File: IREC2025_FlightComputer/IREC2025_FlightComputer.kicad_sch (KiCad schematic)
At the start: 36 parts, among them J1 Molex Microfit, U1 STM32U575VGTx, U2 TPS62153, U3 LP5912Q3.3DRVRQ1

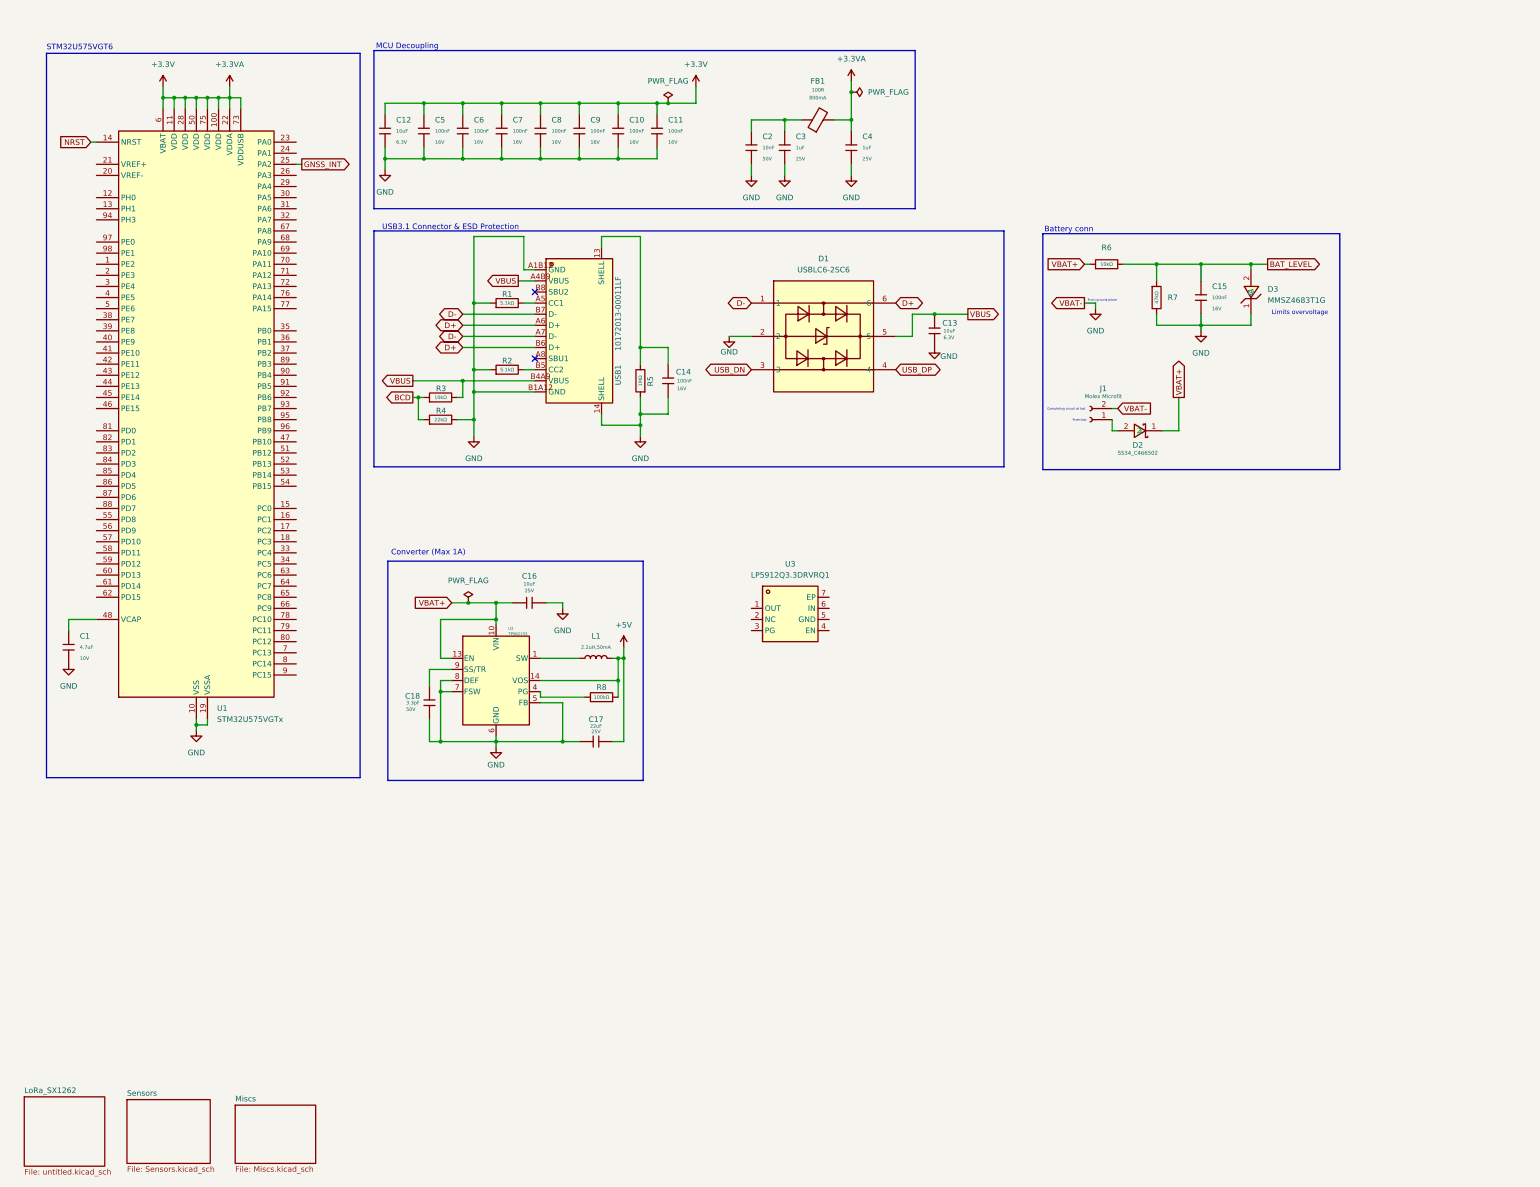
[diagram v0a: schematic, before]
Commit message: Schematics
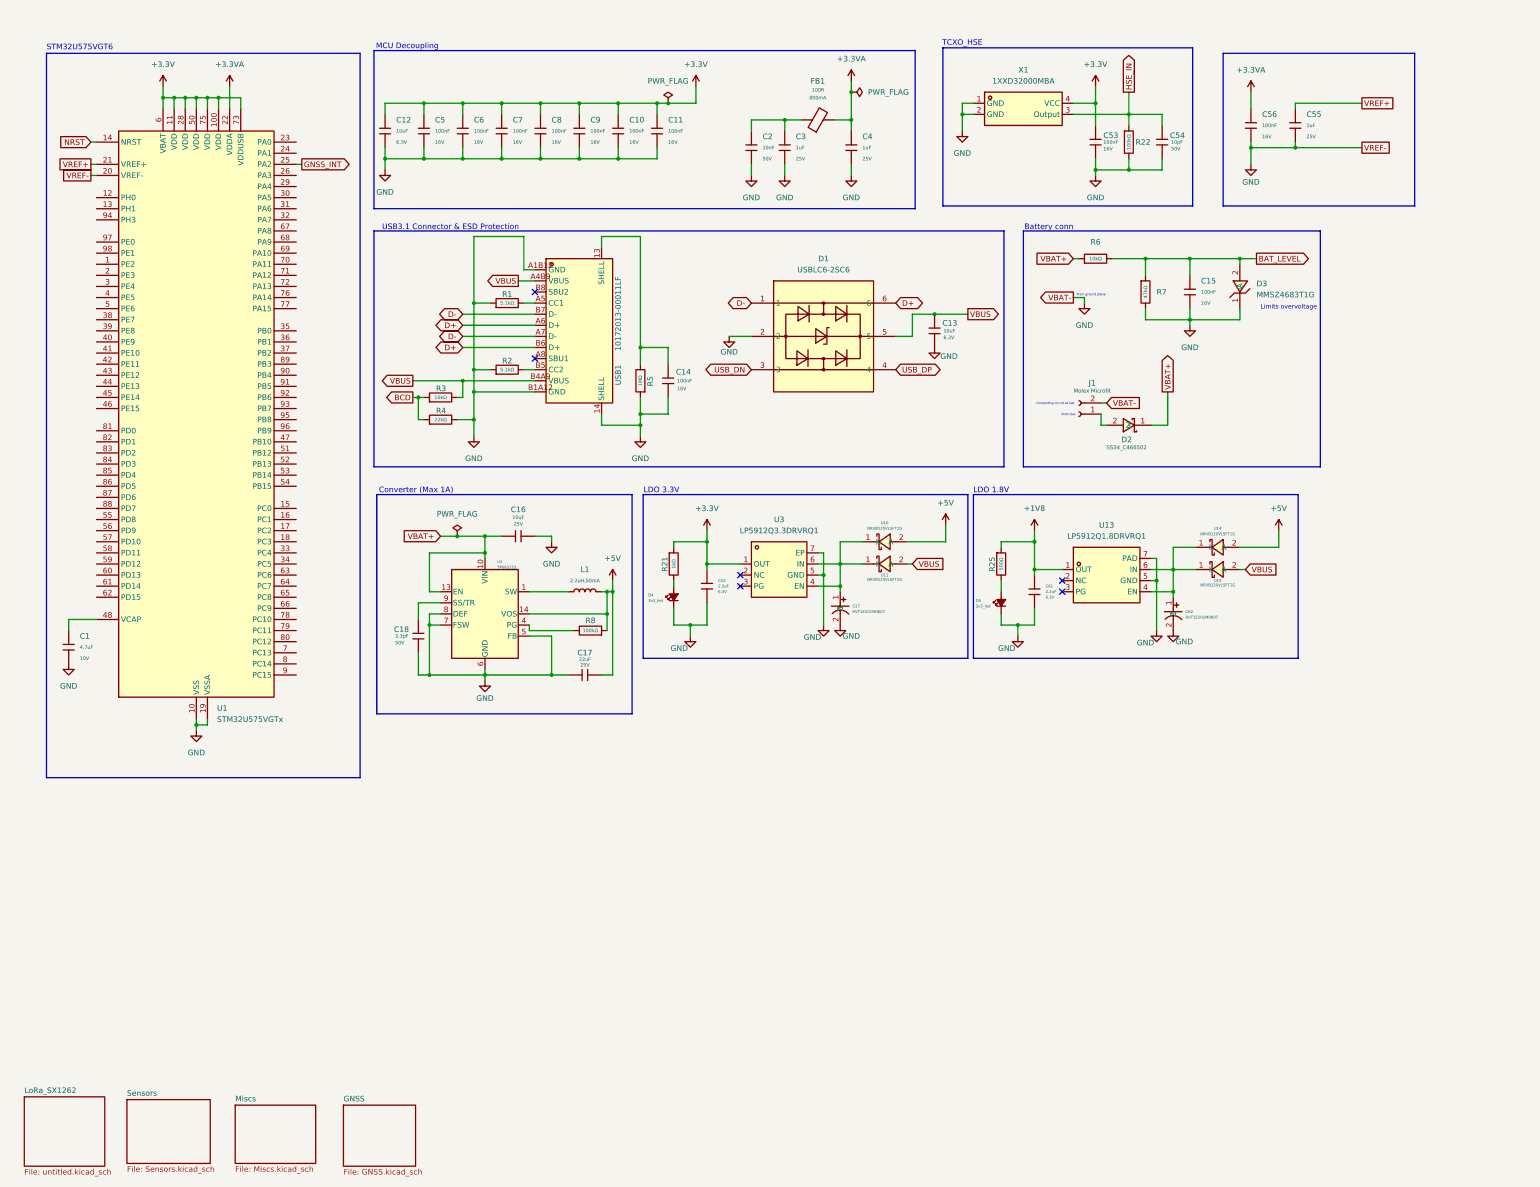
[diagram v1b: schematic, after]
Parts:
- added C27, C62: RVT1E101M0607, EasyEDA:CAP-SMD_BD6.3-L6.6-W6.6-LS7.2-R-RD, symbol EasyEDA:RVT1E101M0607
- added C52, C61: 2.2uF, PCM_JLCPCB:C_0402, symbol PCM_JLCPCB-Capacitors:0402,2.2uF
- added C53, C56: 100nF, PCM_JLCPCB:C_0402, symbol PCM_JLCPCB-Capacitors:0402,100nF
- added C54: 10pF, PCM_JLCPCB:C_0402, symbol PCM_JLCPCB-Capacitors:0402,10pF
- added C55: 1uF, PCM_JLCPCB:C_0402, symbol PCM_JLCPCB-Capacitors:0402,1uF
- added D4, D5: 3v3_led, LED_SMD:LED_0805_2012Metric, symbol Device:LED_Small_Filled
- added R21: 1kΩ, PCM_JLCPCB:R_0805, symbol PCM_JLCPCB-Resistors:0805,1kΩ
- added R22: 100kΩ, PCM_JLCPCB:R_0402, symbol PCM_JLCPCB-Resistors:0402,100kΩ
- added R25: 500Ω, PCM_JLCPCB:R_0805, symbol PCM_JLCPCB-Resistors:0805,1kΩ
- added U10, U11, U14, U15: NRVB120VLSFT1G, EasyEDA:SOD-123_L2.7-W1.6-LS3.7-RD-1, symbol EasyEDA:NRVB120VLSFT1G
- added U13: LP5912Q1.8DRVRQ1, EasyEDA:WSON-6_L2.0-W2.0-P0.65-BL-EP, symbol EasyEDA:LP5912Q1.8DRVRQ1
- added X1: 1XXD32000MBA, EasyEDA:OSC-SMD_4P-L2.0-W1.6-BL_1XXD, symbol EasyEDA:1XXD32000MBA
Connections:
- net +3.3V: now also U3.1 (OUT), C52.1, C53.1, R21.1, X1.4 (VCC); no longer C4.1, FB1.2, U1.22 (VDDA)
- net +5V: now also U10.2 (A), U14.2 (A)
- net GND: now also U1.20 (VREF-), U3.5 (GND), U3.7 (EP), C27.2, C52.2, C53.2, C54.2, C55.2, C56.2, C61.2, C62.2, D4.1 (K), D5.1 (K), R22.2, U13.5 (GND), U13.7 (PAD), X1.1 (GND), X1.2 (GND)
- net VBUS: now also U11.2 (A), U15.2 (A)
- net at U3.4 (EN): now also U3.6 (IN), C27.1, U10.1 (K), U11.1 (K)
- net VREF+: now reaches U1.21 (VREF+)
- net VREF+: now also C55.1
- new net: D4.2 (A), R21.2
- new net: D5.2 (A), R25.2
- new net: C62.1, U13.4 (EN), U13.6 (IN), U14.1 (K), U15.1 (K)
- new net +1V8: C61.1, R25.1, U13.1 (OUT)
- new net +3.3VA: C4.1, C56.1, FB1.2, U1.22 (VDDA)
- new net HSE_IN: C54.1, R22.1, X1.3 (Output)
- no-connect marks 2 -> 6
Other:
- added sheet GNSS (GNSS.kicad_sch)
- note added: "LDO 1.8V"
- note added: "LDO 3.3V"
- note added: "TCXO_HSE"
- moved on the sheet: C15, C16, C17, C18, D2, D3, J1, L1, R6, R7, R8, U2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

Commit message: update
21/3/2025
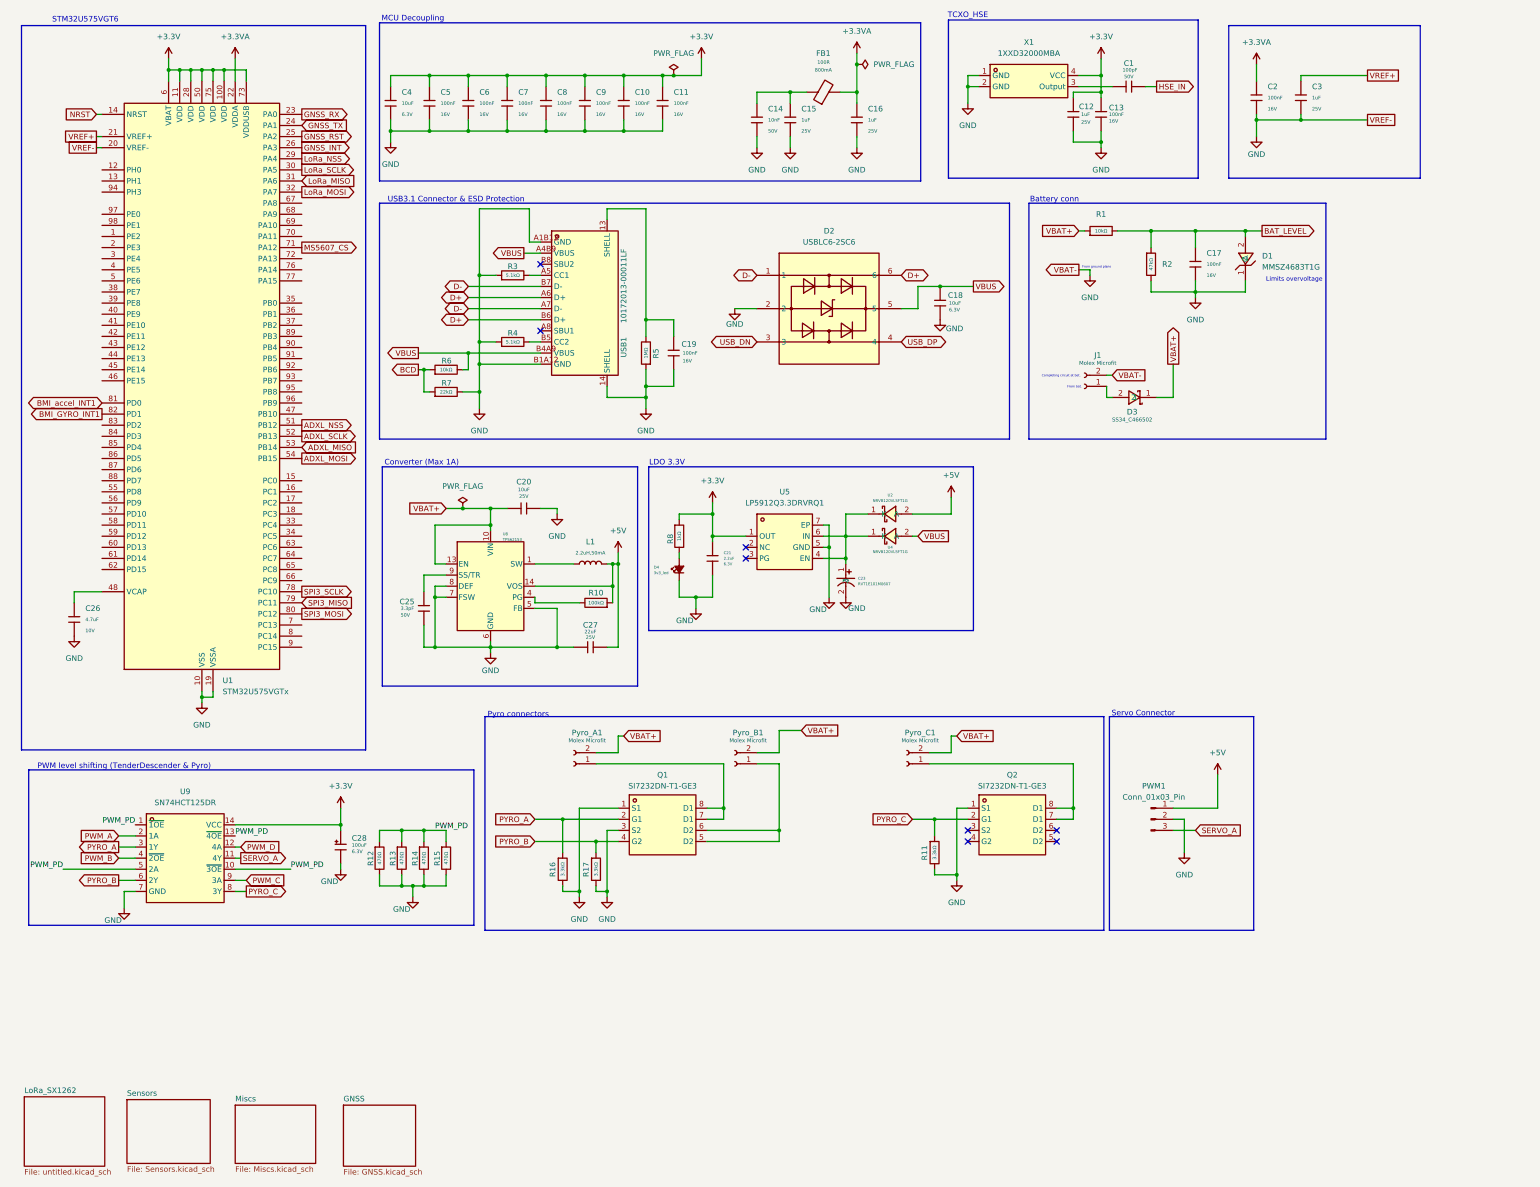
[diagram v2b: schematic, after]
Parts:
- removed C54: 10pF, PCM_JLCPCB:C_0402, symbol PCM_JLCPCB-Capacitors:0402,10pF
- removed C61: 2.2uF, PCM_JLCPCB:C_0402, symbol PCM_JLCPCB-Capacitors:0402,2.2uF
- removed C62: RVT1E101M0607, EasyEDA:CAP-SMD_BD6.3-L6.6-W6.6-LS7.2-R-RD, symbol EasyEDA:RVT1E101M0607
- removed D5: 3v3_led, LED_SMD:LED_0805_2012Metric, symbol Device:LED_Small_Filled
- removed R22: 100kΩ, PCM_JLCPCB:R_0402, symbol PCM_JLCPCB-Resistors:0402,100kΩ
- removed R25: 500Ω, PCM_JLCPCB:R_0805, symbol PCM_JLCPCB-Resistors:0805,1kΩ
- removed U13: LP5912Q1.8DRVRQ1, EasyEDA:WSON-6_L2.0-W2.0-P0.65-BL-EP, symbol EasyEDA:LP5912Q1.8DRVRQ1
- removed U14, U15: NRVB120VLSFT1G, EasyEDA:SOD-123_L2.7-W1.6-LS3.7-RD-1, symbol EasyEDA:NRVB120VLSFT1G
- added C1: 100pF, PCM_JLCPCB:C_0402, symbol PCM_JLCPCB-Capacitors:0402,100pF
- added C12: 1uF, PCM_JLCPCB:C_0402, symbol PCM_JLCPCB-Capacitors:0402,1uF
- added C28: 100uF, PCM_JLCPCB:C_CASE-B-3528-21(mm), symbol PCM_JLCPCB-Capacitors:CASE-B-3528-21(mm),100uF
- added PWM1: Conn_01x03_Pin, Connector_Molex:Molex_Micro-Fit_3.0_43650-0315_1x03_P3.00mm_Vertical, symbol Connector:Conn_01x03_Pin
- added Pyro_A1, Pyro_B1, Pyro_C1: Molex Microfit, Connector_Molex:Molex_Micro-Fit_3.0_43650-0215_1x02_P3.00mm_Vertical, symbol Connector:Conn_01x02_Socket
- added Q1, Q2: SI7232DN-T1-GE3, EasyEDA:POWER-1212-8_L3.3-W3.3-P0.66-LS3.3-BL, symbol EasyEDA:SI7232DN-T1-GE3
- added R11, R16, R17: 3.3kΩ, PCM_JLCPCB:R_0402, symbol PCM_JLCPCB-Resistors:0402,3.3kΩ
- added R12, R13, R14, R15: 470Ω, PCM_JLCPCB:R_0402, symbol PCM_JLCPCB-Resistors:0402,470Ω
- added U9: SN74HCT125DR, EasyEDA:SOIC-14_L8.7-W3.9-P1.27-LS6.0-BL, symbol EasyEDA:SN74HCT125DR
- J1: footprint (none) -> Connector_Molex:Molex_Micro-Fit_3.0_43650-0215_1x02_P3.00mm_Vertical
- renumbered C53 to C13, C2 to C14, C3 to C15, C4 to C16, C15 to C17, C13 to C18, C14 to C19, C56 to C2, C16 to C20, C52 to C21, C27 to C23, C18 to C25, C1 to C26, C17 to C27, C55 to C3, C12 to C4, D3 to D1, D1 to D2, D2 to D3, R6 to R1, R8 to R10, R7 to R2, R1 to R3, R2 to R4, R3 to R6, R4 to R7, R21 to R8, U10 to U2, U11 to U4, U3 to U5, U2 to U8
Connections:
- net +3.3V: now also C12.1, C28.1, U9.14 (VCC)
- net +5V: now also PWM1.1 (Pin_1)
- net GND: now also C12.2, C28.2, PWM1.2 (Pin_2), Q1.1 (S1), Q1.3 (S2), Q2.1 (S1), R11.2, R12.2, R13.2, R14.2, R15.2, R16.2, R17.2, U9.7 (GND)
- net GNSS_INT: now also U1.26 (PA3); no longer U1.25 (PA2)
- net HSE_IN: now also C1.2; no longer X1.3 (Output)
- net VBAT+: now also Pyro_A1.2 (Pin_2), Pyro_B1.2 (Pin_2), Pyro_C1.2 (Pin_2)
- net GNSS_RX: now reaches U1.23 (PA0)
- net GNSS_TX: now reaches U1.24 (PA1)
- net LoRa_NSS: now reaches U1.29 (PA4)
- net LoRa_SCLK: now reaches U1.30 (PA5)
- net LoRa_MISO: now reaches U1.31 (PA6)
- net LoRa_MOSI: now reaches U1.32 (PA7)
- net ADXL_NSS: now reaches U1.51 (PB12)
- net ADXL_SCLK: now reaches U1.52 (PB13)
- net ADXL_MISO: now reaches U1.53 (PB14)
- net ADXL_MOSI: now reaches U1.54 (PB15)
- net MS5607_CS: now reaches U1.71 (PA12)
- net SPI3_SCLK: now reaches U1.78 (PC10)
- net SPI3_MISO: now reaches U1.79 (PC11)
- net SPI3_MOSI: now reaches U1.80 (PC12)
- net BMI_accel_INT1: now reaches U1.81 (PD0)
- net BMI_GYRO_INT1: now reaches U1.82 (PD1)
- new net: C1.1, X1.3 (Output)
- new net: Pyro_C1.1 (Pin_1), Q2.7 (D1), Q2.8 (D1)
- new net: Pyro_A1.1 (Pin_1), Q1.7 (D1), Q1.8 (D1)
- new net: Pyro_B1.1 (Pin_1), Q1.5 (D2), Q1.6 (D2)
- new net GNSS_RST: U1.25 (PA2)
- new net PWM_A: U9.2 (1A)
- new net PWM_B: U9.4 (~{2OE})
- new net PWM_C: U9.9 (3A)
- new net PWM_D: U9.12 (4A)
- new net PWM_PD: R12.1, R13.1, R14.1, R15.1, U9.1 (~{1OE}), U9.10 (~{3OE}), U9.13 (~{4OE}), U9.5 (2A)
- new net PYRO_A: Q1.2 (G1), R16.1, U9.3 (1Y)
- new net PYRO_B: Q1.4 (G2), R17.1, U9.6 (2Y)
- new net PYRO_C: Q2.2 (G1), R11.1, U9.8 (3Y)
- new net SERVO_A: PWM1.3 (Pin_3), U9.11 (4Y)
- no-connect marks 6 -> 8
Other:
- note added: "PWM level shifting (TenderDescender & Pyro)"
- note added: "Pyro connectors"
- note added: "Servo Connector"
- note removed: "LDO 1.8V"
- moved on the sheet: C10, C11, C13, C14, C15, C16, C17, C18, C19, C2, C20, C21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

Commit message: Updated 22/3/2025
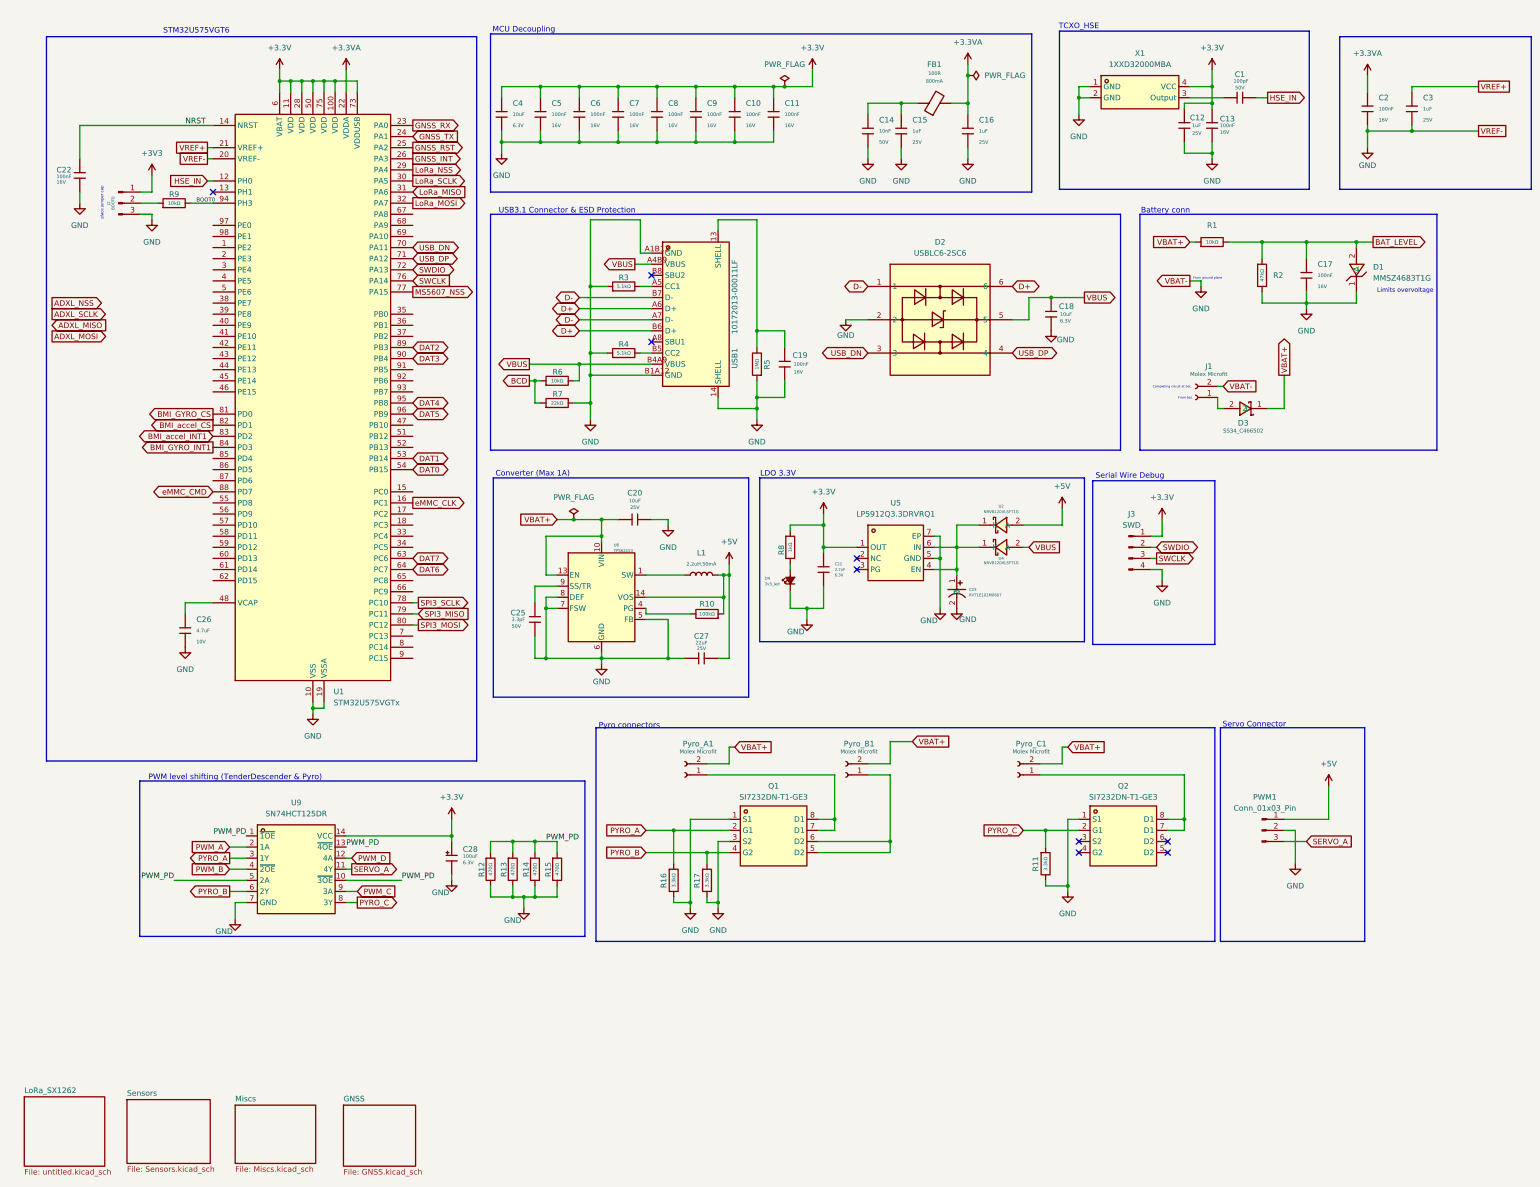
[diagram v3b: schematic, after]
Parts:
- added C22: 100nF, PCM_JLCPCB:C_0402, symbol PCM_JLCPCB-Capacitors:0402,100nF
- added J2: BOOT0, Connector_PinHeader_2.54mm:PinHeader_1x03_P2.54mm_Vertical, symbol Connector:Conn_01x03_Pin
- added J3: SWD, Connector_PinHeader_2.54mm:PinHeader_1x04_P2.54mm_Vertical, symbol Connector:Conn_01x04_Pin
- added R9: 10kΩ, PCM_JLCPCB:R_0402, symbol PCM_JLCPCB-Resistors:0402,10kΩ
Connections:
- net MS5607_CS is gone; now on net USB_DP: U1.71 (PA12)
- net +3.3V: now also J3.1 (Pin_1)
- net ADXL_MISO: no longer U1.53 (PB14)
- net ADXL_MOSI: no longer U1.54 (PB15)
- net ADXL_NSS: no longer U1.51 (PB12)
- net ADXL_SCLK: no longer U1.52 (PB13)
- net BMI_GYRO_INT1: now also U1.84 (PD3); no longer U1.82 (PD1)
- net BMI_accel_INT1: now also U1.83 (PD2); no longer U1.81 (PD0)
- net GND: now also C22.2, J2.3 (Pin_3), J3.4 (Pin_4)
- net HSE_IN: now also U1.12 (PH0)
- net NRST: now also C22.1
- net USB_DN: now also U1.70 (PA11)
- net eMMC_CLK: now reaches U1.16 (PC1)
- net DAT7: now reaches U1.63 (PC6)
- net DAT6: now reaches U1.64 (PC7)
- net SWDIO: now reaches U1.72 (PA13)
- net SWDIO: now also J3.2 (Pin_2)
- net SWCLK: now reaches U1.76 (PA14)
- net SWCLK: now also J3.3 (Pin_3)
- net MS5607_NSS: now reaches U1.77 (PA15)
- net eMMC_CMD: now reaches U1.88 (PD7)
- net DAT2: now reaches U1.89 (PB3)
- net DAT3: now reaches U1.90 (PB4)
- net BOOT0: now reaches U1.94 (PH3)
- net BOOT0: now also R9.2
- net DAT4: now reaches U1.95 (PB8)
- net DAT5: now reaches U1.96 (PB9)
- new net: J2.2 (Pin_2), R9.1
- new net +3V3: J2.1 (Pin_1)
- new net BMI_GYRO_CS: U1.81 (PD0)
- new net BMI_accel_CS: U1.82 (PD1)
- new net DAT0: U1.54 (PB15)
- new net DAT1: U1.53 (PB14)
- no-connect marks 8 -> 9
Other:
- note added: "Serial Wire Debug"
- note added: "place jumper cap"
- moved on the sheet: C1, C10, C11, C12, C13, C14, C15, C16, C17, C18, C19, C2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
